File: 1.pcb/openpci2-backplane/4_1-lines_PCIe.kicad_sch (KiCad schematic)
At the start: 24 parts, among them J10 10018784-10210TLF, J11 10018784-10210TLF, J12 10018784-10210TLF, J5 1-2199230-6, J6 1-2199230-6, J7 10018784-10210TLF, J8 1-2199230-6, J9 1-2199230-6

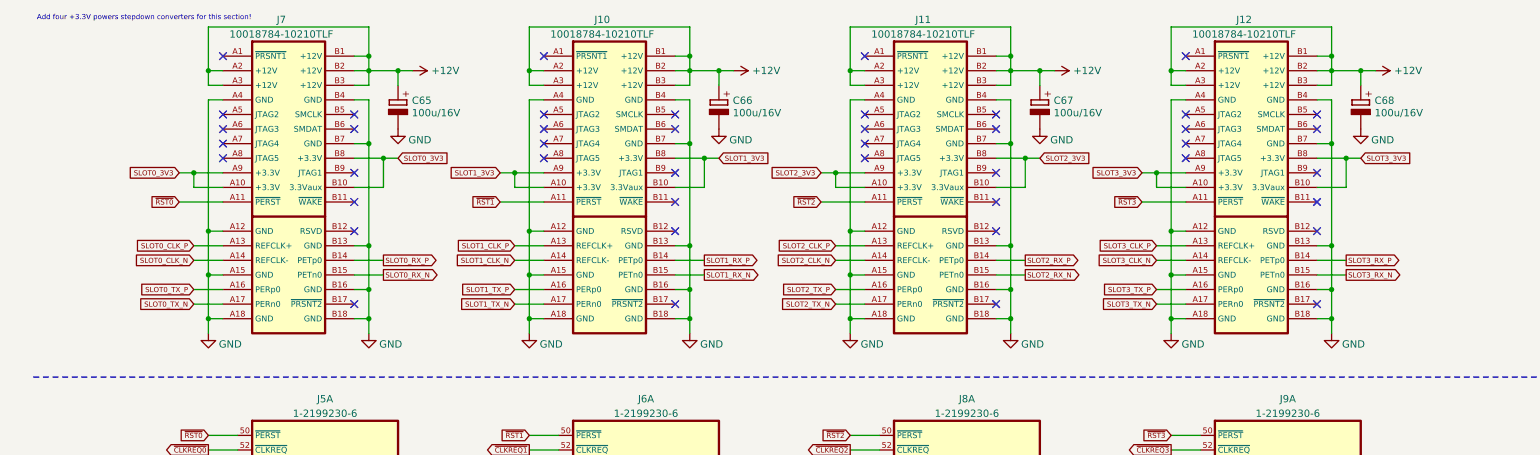
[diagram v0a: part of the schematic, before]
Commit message: PCIe connectors update
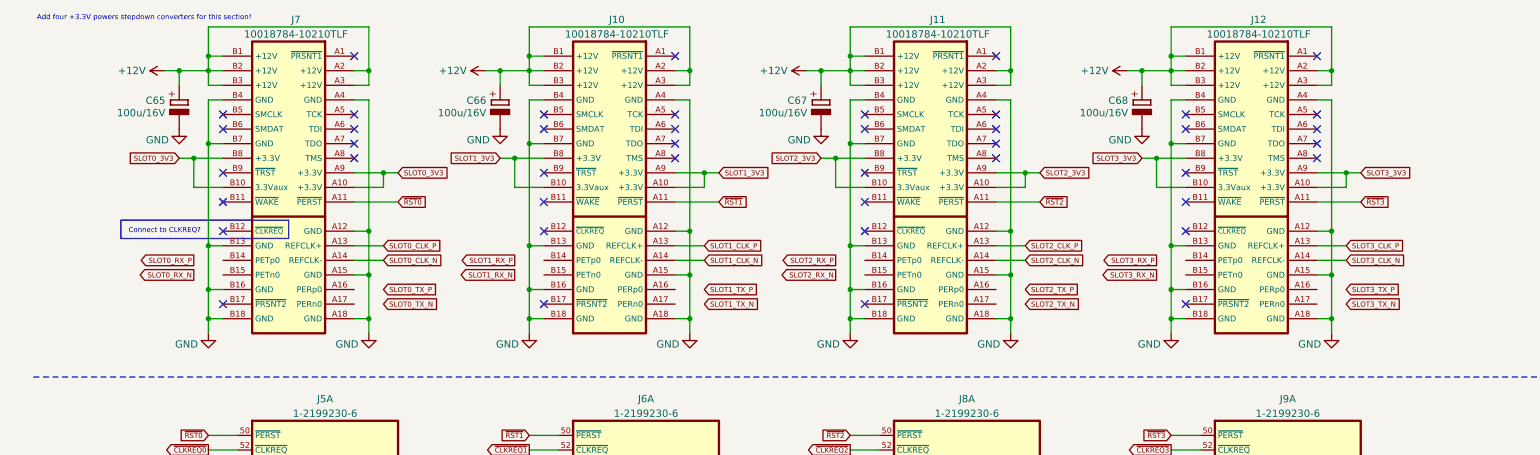
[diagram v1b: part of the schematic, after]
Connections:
- net SLOT0_RX_N: no longer J7.B15 (PETn0)
- net SLOT0_RX_P: no longer J7.B14 (PETp0)
- net SLOT0_TX_N: no longer J7.A17 (PERn0)
- net SLOT0_TX_P: no longer J7.A16 (PERp0)
- net SLOT1_RX_N: no longer J10.B15 (PETn0)
- net SLOT1_RX_P: no longer J10.B14 (PETp0)
- net SLOT1_TX_N: no longer J10.A17 (PERn0)
- net SLOT1_TX_P: no longer J10.A16 (PERp0)
- net SLOT2_RX_N: no longer J11.B15 (PETn0)
- net SLOT2_RX_P: no longer J11.B14 (PETp0)
- net SLOT2_TX_N: no longer J11.A17 (PERn0)
- net SLOT2_TX_P: no longer J11.A16 (PERp0)
- net SLOT3_RX_N: no longer J12.B15 (PETn0)
- net SLOT3_RX_P: no longer J12.B14 (PETp0)
- net SLOT3_TX_N: no longer J12.A17 (PERn0)
- net SLOT3_TX_P: no longer J12.A16 (PERp0)
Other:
- note added: "Connect to CLKREQ?"
- moved on the sheet: C65, C66, C67, C68
